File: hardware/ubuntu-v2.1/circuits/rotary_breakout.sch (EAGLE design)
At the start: 29 parts, among them SW2 SWITCH-ALPS_EC12E_SW, SW3 SWITCH-ALPS_EC12E_SW, SW4 SWITCH-ALPS_EC12E_SW, SW5 SWITCH-ALPS_EC12E_SW

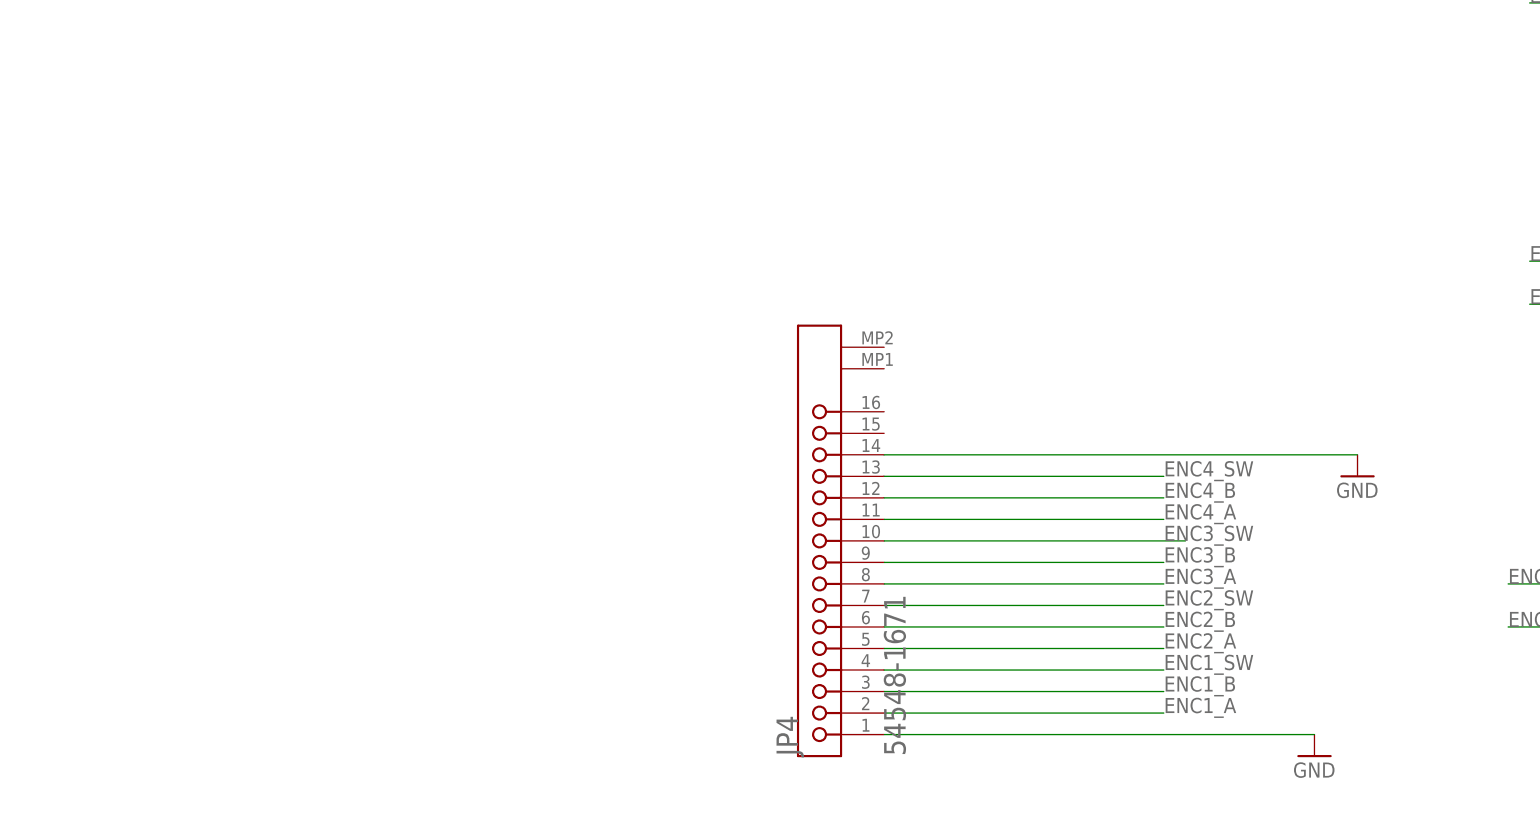
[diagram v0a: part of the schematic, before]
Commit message: Add files via upload
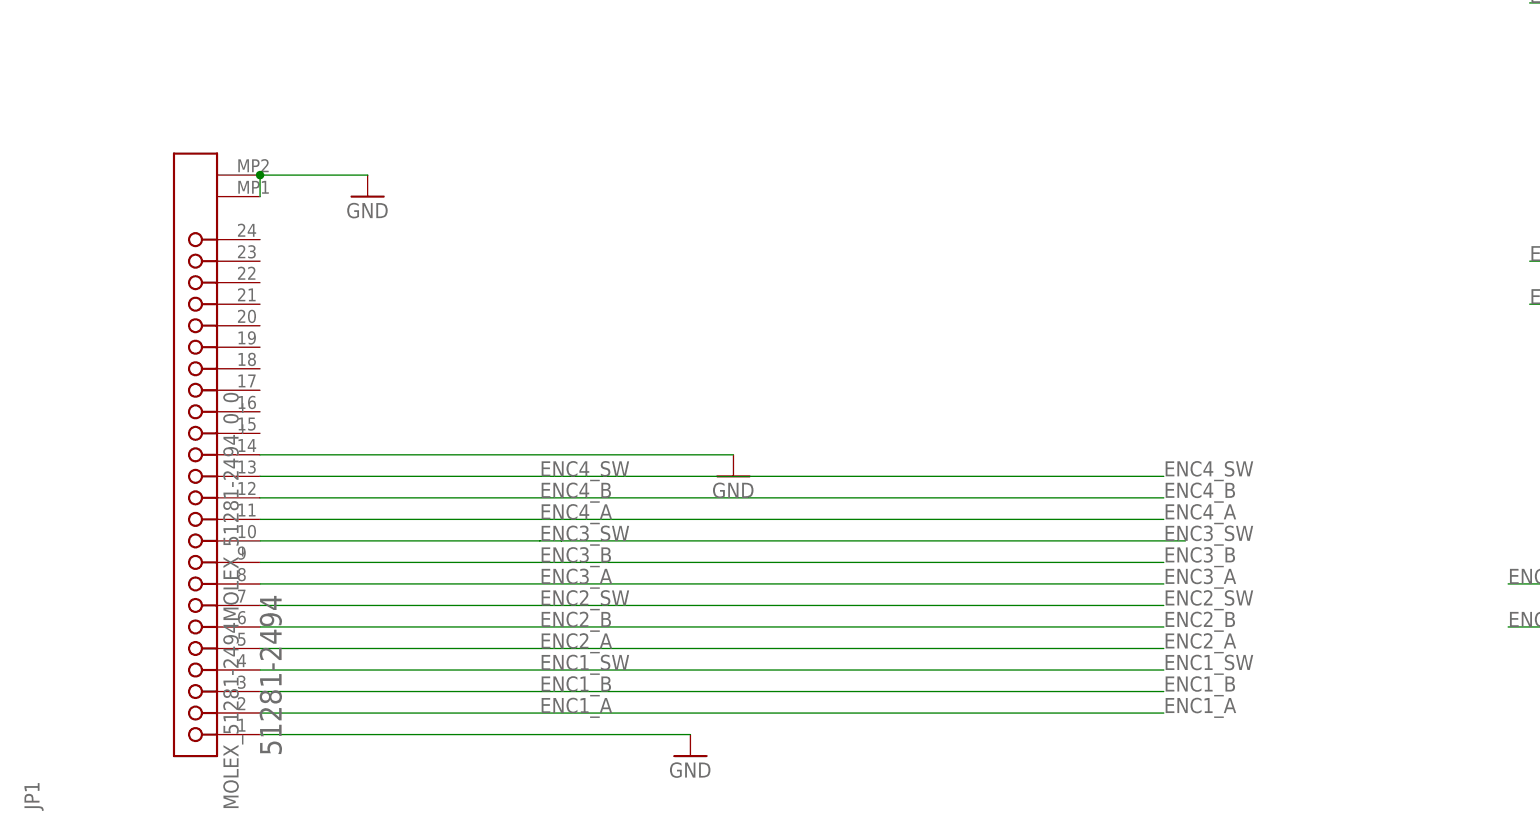
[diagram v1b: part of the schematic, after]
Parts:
- removed JP4: MOLEX_54548-1671MOLEX_54548-1671_0_0, Molex - 54548-1671:MOLEX_54548-1671MOLEX_54548-1671_0_0
- added JP1: MOLEX_51281-2494MOLEX_51281-2494_0_0, Molex - 51281-2494:MOLEX_51281-2494MOLEX_51281-2494_0_0
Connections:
- net ENC1_A: now also JP1.2; no longer JP4.2
- net ENC1_B: now also JP1.3; no longer JP4.3
- net ENC1_SW: now also JP1.4; no longer JP4.4
- net ENC2_A: now also JP1.5; no longer JP4.5
- net ENC2_B: now also JP1.6; no longer JP4.6
- net ENC2_SW: now also JP1.7; no longer JP4.7
- net ENC3_A: now also JP1.8; no longer JP4.8
- net ENC3_B: now also JP1.9; no longer JP4.9
- net ENC3_SW: now also JP1.10; no longer JP4.10
- net ENC4_A: now also JP1.11; no longer JP4.11
- net ENC4_B: now also JP1.12; no longer JP4.12
- net ENC4_SW: now also JP1.13; no longer JP4.13
- net GND: now also JP1.1, JP1.14, JP1.MP1, JP1.MP2; no longer JP4.1, JP4.14
